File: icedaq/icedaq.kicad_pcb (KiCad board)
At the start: 2 copper layers, 53 parts, among them J1 analog outputs, J2 analog inputs, P1 UART, U1 REG12, U2 iCE40HX1K-VQ100, U3 RPi, U4 oscillator4, U5 ADC082S021, U6 ADC082S021, U7 MCP6004

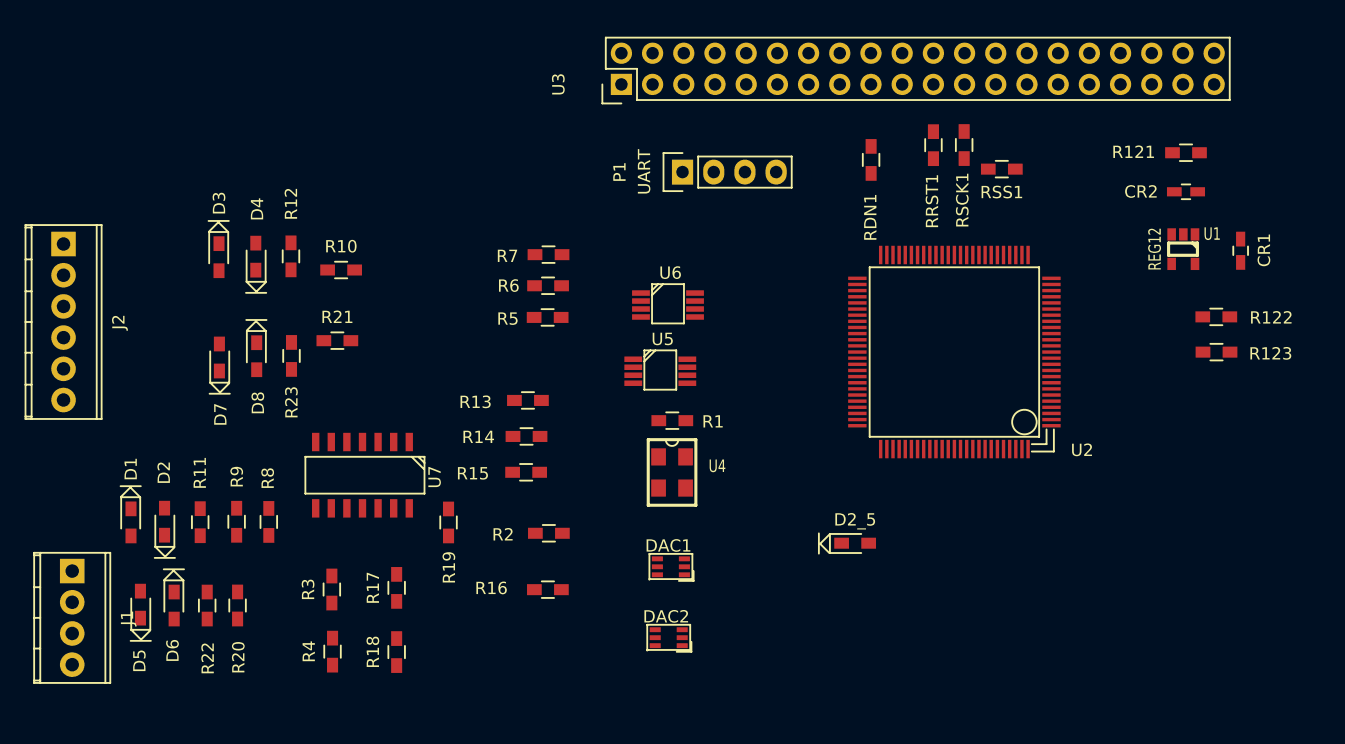
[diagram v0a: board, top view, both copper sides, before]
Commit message: icedaq layout
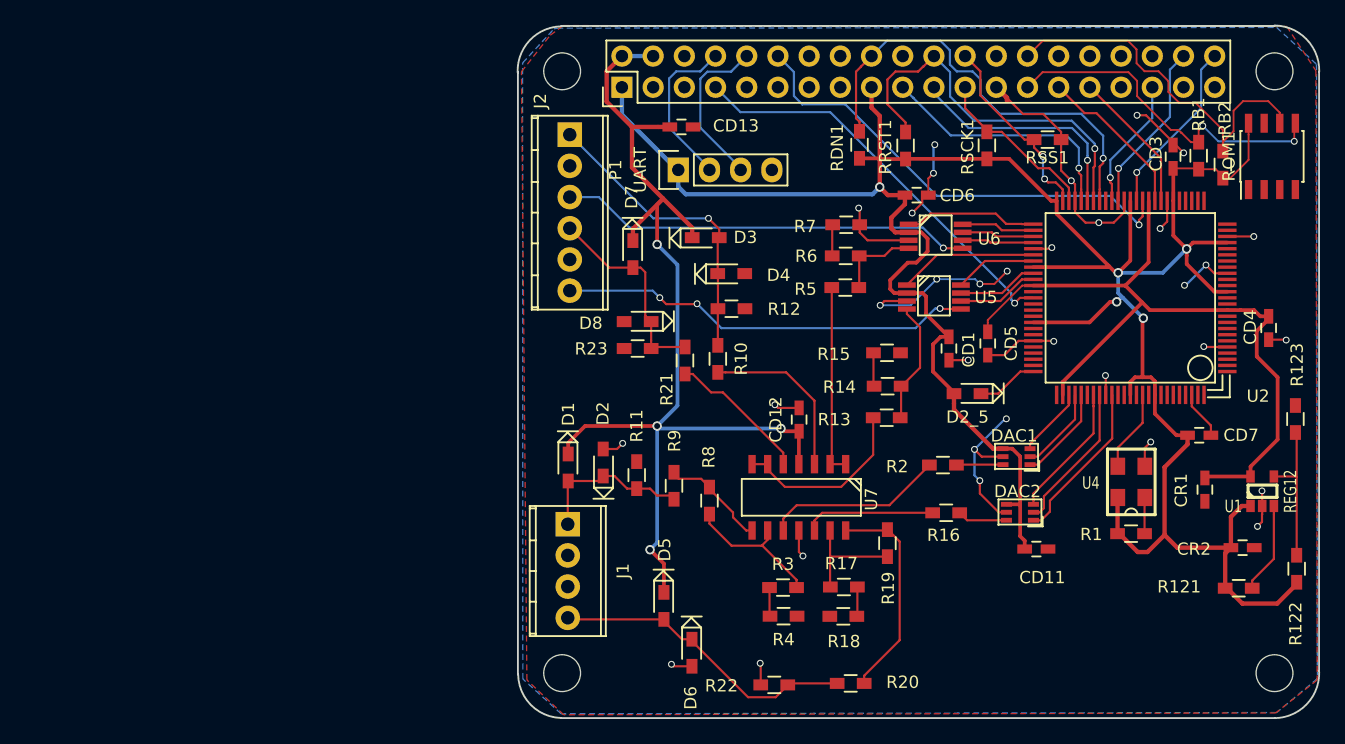
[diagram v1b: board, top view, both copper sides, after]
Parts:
- added CD1: C_Small, Capacitors_SMD:C_0603_HandSoldering, F.Cu at (171.6, 81.3)
- added CD11: C_Small, Capacitors_SMD:C_0603_HandSoldering, F.Cu at (178.7, 97.6)
- added CD12: C_Small, Capacitors_SMD:C_0603_HandSoldering, F.Cu at (159.4, 87.1)
- added CD13: C_Small, Capacitors_SMD:C_0603_HandSoldering, F.Cu at (149.8, 63.2)
- added CD3: C_Small, Capacitors_SMD:C_0603_HandSoldering, F.Cu at (189.9, 65.7)
- added CD4: C_Small, Capacitors_SMD:C_0603_HandSoldering, F.Cu at (197.7, 79.6)
- added CD5: C_Small, Capacitors_SMD:C_0603_HandSoldering, F.Cu at (174.8, 80.9)
- added CD6: C_Small, Capacitors_SMD:C_0603_HandSoldering, F.Cu at (169.0, 68.8)
- added CD7: C_Small, Capacitors_SMD:C_0603_HandSoldering, F.Cu at (192.0, 88.3)
- added RB1: 3.9k, Resistors_SMD:R_0603_HandSoldering, F.Cu at (192.0, 65.6)
- added RB2: 3.9k, Resistors_SMD:R_0603_HandSoldering, F.Cu at (193.9, 66.3)
- added REF**: MountingHole_3mm, Mounting_Holes:MountingHole_3mm, F.Cu at (140.1, 58.7)
- added REF**: MountingHole_3mm, Mounting_Holes:MountingHole_3mm, F.Cu at (198.1, 58.7)
- added REF**: MountingHole_3mm, Mounting_Holes:MountingHole_3mm, F.Cu at (198.1, 107.7)
- added REF**: MountingHole_3mm, Mounting_Holes:MountingHole_3mm, F.Cu at (140.1, 107.7)
- added ROM1: CAT24C, Housings_SOIC:SOIC-8_3.9x4.9mm_Pitch1.27mm, F.Cu at (197.9, 65.6)
- moved R20 50.3 mm to (163.6, 108.5), turned to 0 degrees
- moved R22 46.6 mm to (157.4, 108.7), turned to 0 degrees
- moved D5 42.6 mm to (148.4, 102.2), turned to 270 degrees
- moved D6 42.3 mm to (150.7, 106.0)
- moved J2 42.2 mm to (140.8, 63.9)
- moved J1 40.5 mm to (140.6, 95.6)
- moved D3 39.7 mm to (151.8, 72.2), turned to 0 degrees
- moved D4 38.7 mm to (153.9, 75.2), turned to 0 degrees
- moved R1 38.5 mm to (186.4, 96.3)
- moved U4 37.4 mm to (186.5, 92.1), turned to 180 degrees
- moved R4 36.8 mm to (158.2, 103.1), turned to 180 degrees
- moved R3 36.7 mm to (158.1, 100.7), turned to 0 degrees
- moved R18 36.5 mm to (163.0, 103.1), turned to 0 degrees
- moved R17 36.4 mm to (163.1, 100.7), turned to 180 degrees
- moved R12 36.1 mm to (153.9, 78.0), turned to 180 degrees
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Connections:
- R1 pad 1: +3V3 -> Net-(R1-Pad1)
- R1 pad 2: Net-(R1-Pad2) -> +3V3
- U2 pad 30: /GCLK2 -> (no net)
- U2 pad 37: /MISO1 -> /SCLK1
- U2 pad 41: /SCLK1 -> /MISO1
- U2 pad 63: /Analog/clk -> GCLK2
- U2 pad 65: /Analog/din3 -> (no net)
- U2 pad 66: /Analog/slkc3 -> (no net)
- U2 pad 68: /Analog/sync3 -> (no net)
- U2 pad 71: /Analog/din4 -> (no net)
- U2 pad 72: /Analog/sclk4 -> (no net)
- U2 pad 73: /Analog/sync4 -> (no net)
- U2 pad 78: (no net) -> /Analog/din3
- U2 pad 79: (no net) -> /Analog/slkc3
- U2 pad 80: (no net) -> /Analog/sync3
- U2 pad 82: (no net) -> /Analog/din4
- U2 pad 83: (no net) -> /Analog/sclk4
- U2 pad 85: (no net) -> /Analog/sync4
- U2 pad 90: (no net) -> clk
- U3 pad 27: (no net) -> /ID_SD
- U3 pad 28: (no net) -> /ID_SC
- U3 pad 31: /GCLK2 -> /GCLK0
- U3 pad 7: /GCLK0 -> GCLK2
- U4 pad 1: Net-(R1-Pad2) -> Net-(R1-Pad1)
- U4 pad 3: /Analog/clk -> clk
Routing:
- net +3V3: track 0.00 -> 215.8 mm, vias 0 -> 5
- net GND: track 0.00 -> 107.5 mm, vias 0 -> 33
- net +5V: track 0.00 -> 85.7 mm, vias 0 -> 4
- net +1V2: track 0.00 -> 62.7 mm
- net /SS1: track 0.00 -> 38.3 mm, vias 0 -> 1
- net /CDONE: track 0.00 -> 36.2 mm, vias 0 -> 1
- net /Analog/in4a: track 0.00 -> 33.8 mm, vias 0 -> 3
- net /Analog/in2a: track 0.00 -> 33.7 mm, vias 0 -> 1
- net GCLK2: track 0.00 -> 33.6 mm, vias 0 -> 1
- net /CRST: track 0.00 -> 31.4 mm, vias 0 -> 1
- net /ID_SC: track 0.00 -> 31.3 mm
- net /ID_SD: track 0.00 -> 28.5 mm, vias 0 -> 2
- net /Analog/out4: track 0.00 -> 25.3 mm
- net /Analog/in1: track 0.00 -> 24.9 mm, vias 0 -> 1
- net /MOSI: track 0.00 -> 20.8 mm, vias 0 -> 1
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- added copper zone on B.Cu, net GND
- added copper zone on F.Cu, net GND
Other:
- board outline added: 65.3 x 56.4 mm
- net class Default: clearance 0.2 -> 0.1524; trace_width 0.25 -> 0.1778; via_dia 0.6 -> 0.5588; via_drill 0.4 -> 0.381
- net class Ground added: clearance 0.1524, trace_width 0.1778, via_dia 0.5588, via_drill 0.381
- net class Power added: clearance 0.2032, trace_width 0.3556, via_dia 0.762, via_drill 0.4826
- rule trace_clearance: 0.2 -> 0.1524
- rule trace_min: 0.2 -> 0.1524
- rule via_min_drill: 0.3 -> 0.3302
- rule via_min_size: 0.4 -> 0.508
